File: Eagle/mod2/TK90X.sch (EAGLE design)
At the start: 219 parts, among them IC1 Z80, IC10 74LS365N, IC11 LM1886, IC12 LM1889, IC13 4116, IC14 4116, IC15 4116, IC16 4116, IC17 4116, IC18 4116, IC19 4116, IC2 ROM, IC20 4116, IC21 4416, IC22 4416, IC23 4416, IC24 4416, IC25 74LS00, IC26 74LS00, IC27 74LS32, IC28 74LS04, IC3 ULA TK90, IC4 74LS74, IC5 74LS74, IC6 74LS157, IC7 74LS157, IC8 74LS157, IC9 74LS157, Q1 BC548, Q2 BC548, Q3 BF494, Q4 BC548, Q5 BD139, Q6 BD136, Q7 BC548, Q8 2N4401, X2 POWER

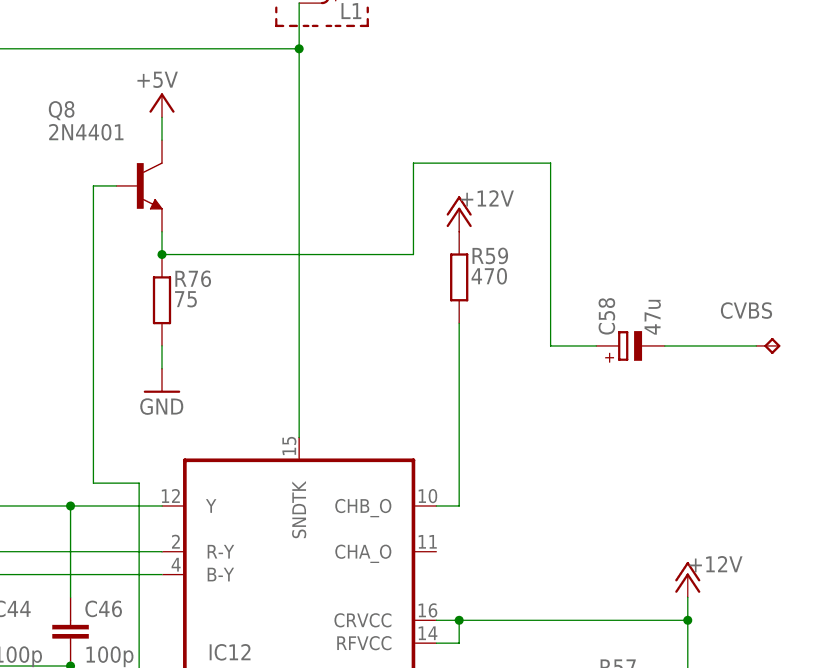
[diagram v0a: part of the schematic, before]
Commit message: Alguns ajustes no mod2
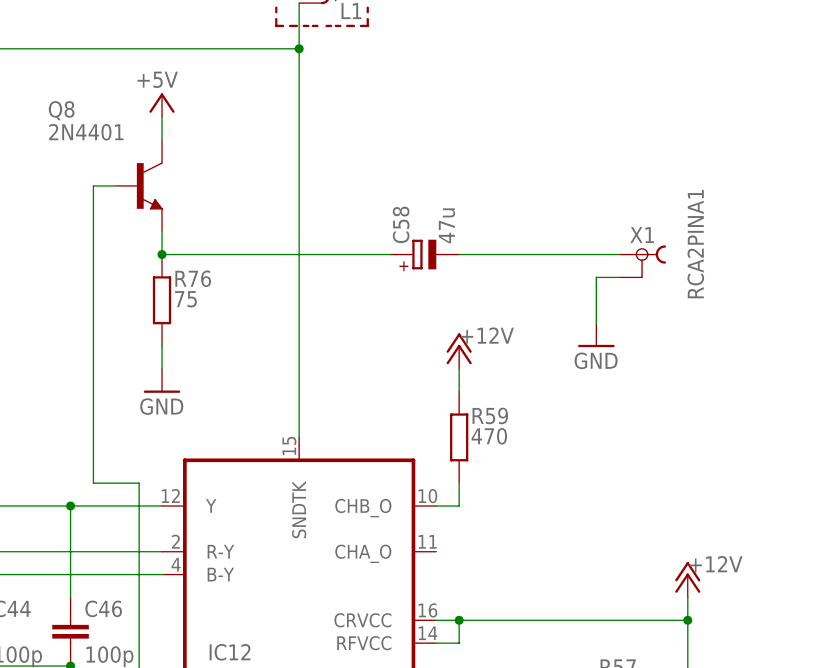
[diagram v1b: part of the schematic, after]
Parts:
- removed CVBS: RF, testpad:TPPAD1-13
- added X1: RCA2PINA1, tk90:RCA2PINA1
- Q8: device transistor-npn:2N4416 -> tk90:2N4401
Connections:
- removed net N$76: C58.-, CVBS.TP
- new net N$74: C58.-, X1.1
- net GND: now also X1.2
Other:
- moved on the sheet: C58, R59
